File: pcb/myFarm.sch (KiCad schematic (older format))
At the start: 10 parts, among them J0 Conn_01x02, J1 LED, J2 SENSOR, J3 SW_LED, J4 RELAY, J5 POWER DRIVE, J6 JUMPER, J7 SW_LED, U1 WeMos_D1_mini, U2 MCP23017_MODULE

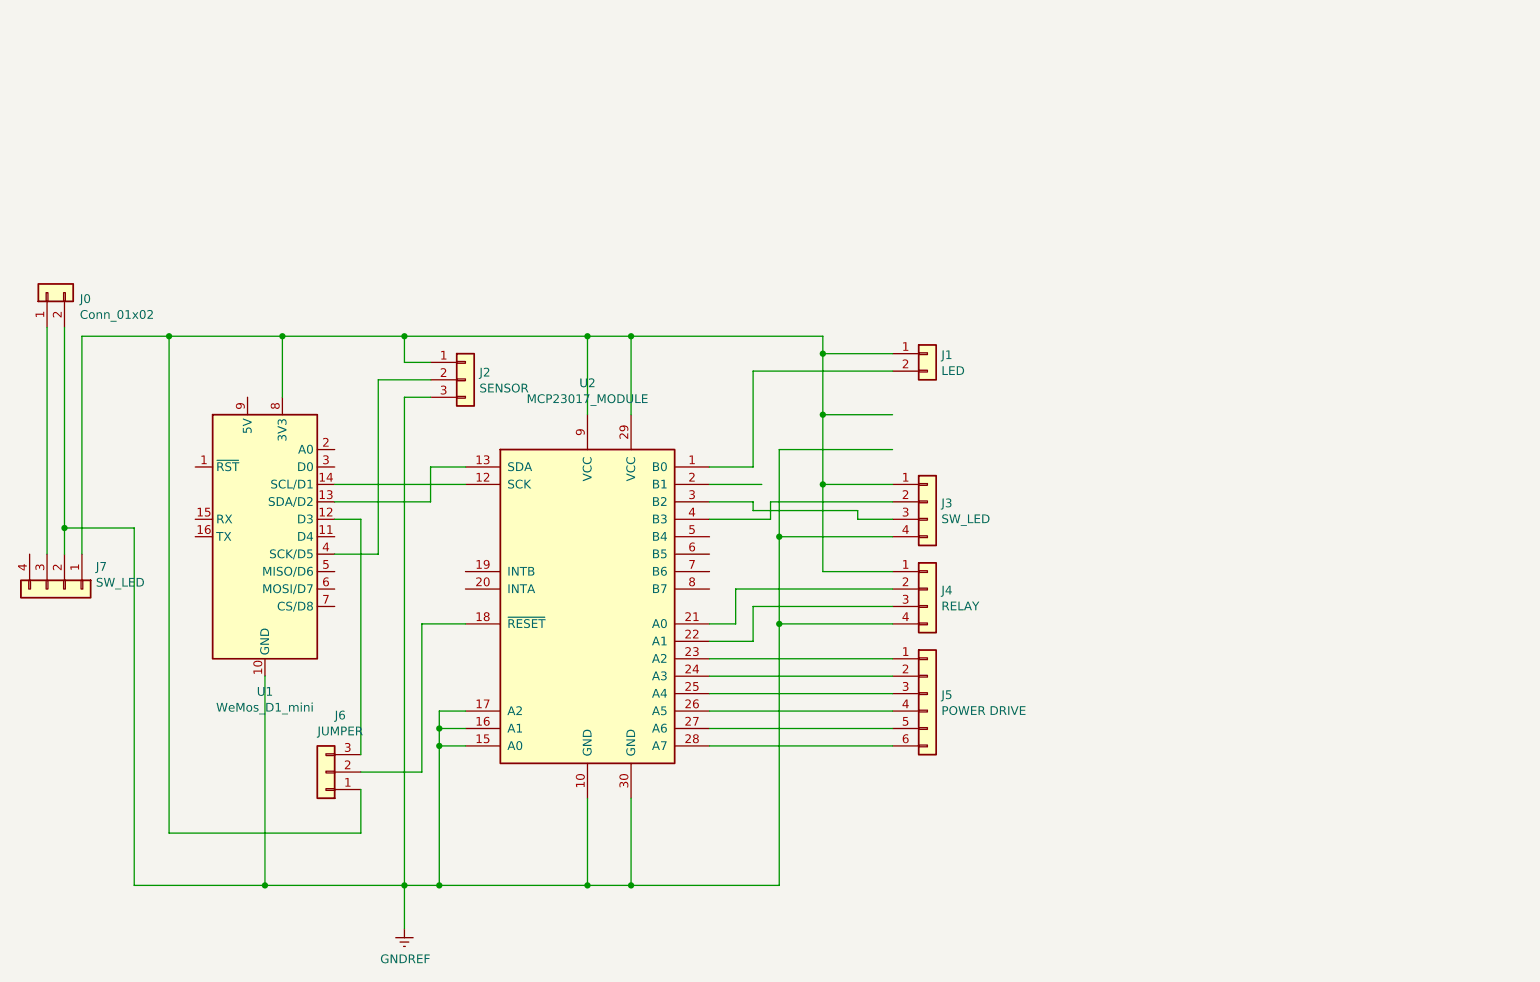
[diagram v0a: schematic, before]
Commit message: update pcb
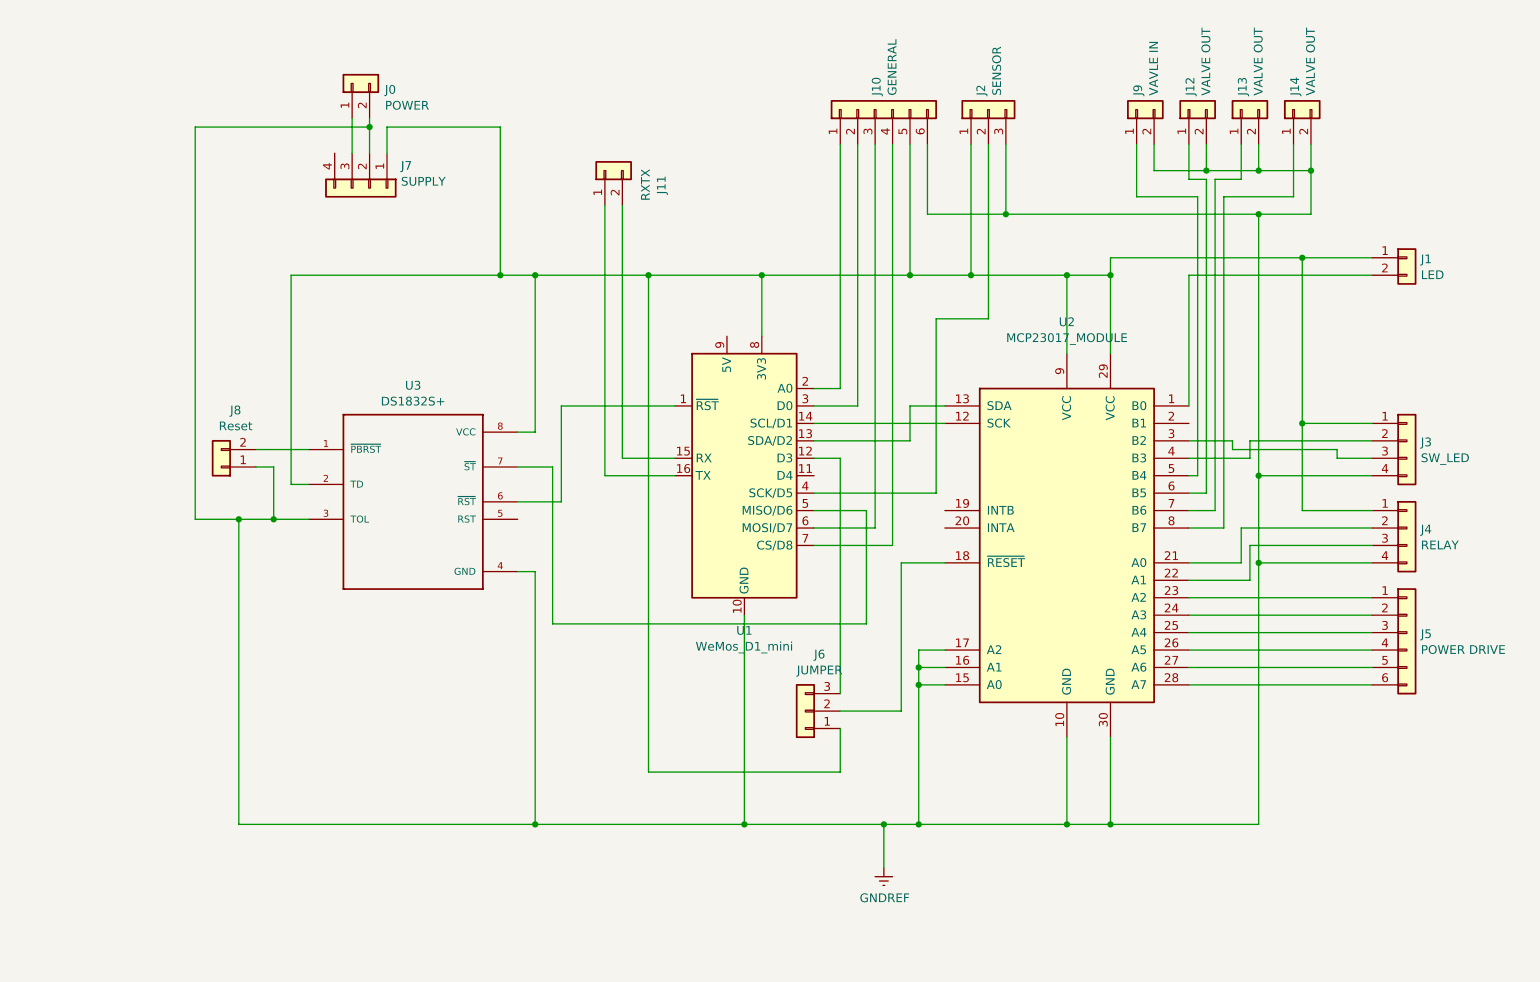
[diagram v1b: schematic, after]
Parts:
- added J10: GENERAL, Connector_PinHeader_2.54mm:PinHeader_1x06_P2.54mm_Vertical, symbol Connector_Generic:Conn_01x06
- added J11: RXTX, Connector_PinHeader_2.54mm:PinHeader_1x02_P2.54mm_Vertical, symbol Connector_Generic:Conn_01x02
- added J12, J13, J14: VALVE OUT, Connector_PinHeader_2.54mm:PinHeader_1x02_P2.54mm_Vertical, symbol Connector_Generic:Conn_01x02
- added J8: Reset, Connector_PinHeader_2.54mm:PinHeader_1x02_P2.54mm_Vertical, symbol Connector_Generic:Conn_01x02
- added J9: VAVLE IN, Connector_PinHeader_2.54mm:PinHeader_1x02_P2.54mm_Vertical, symbol Connector_Generic:Conn_01x02
- added U3: DS1832S+, Package_DIP:DIP-8_W10.16mm, symbol DS1832S_:DS1832S+
- J0: value Conn_01x02 -> POWER
- J7: value SW_LED -> SUPPLY
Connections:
- wire segments 88 -> 150
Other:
- moved on the sheet: J0, J1, J2, J3, J4, J5, J6, J7, U1, U2

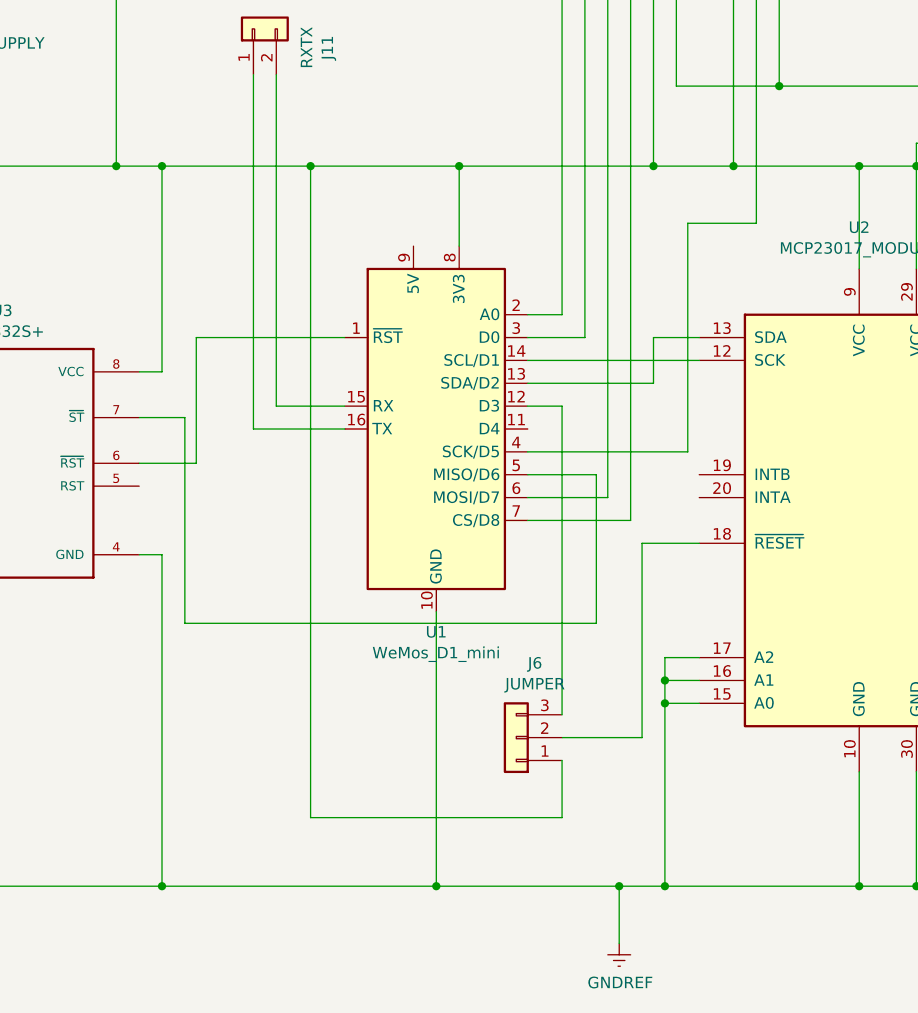
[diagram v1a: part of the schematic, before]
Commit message: update pcb.
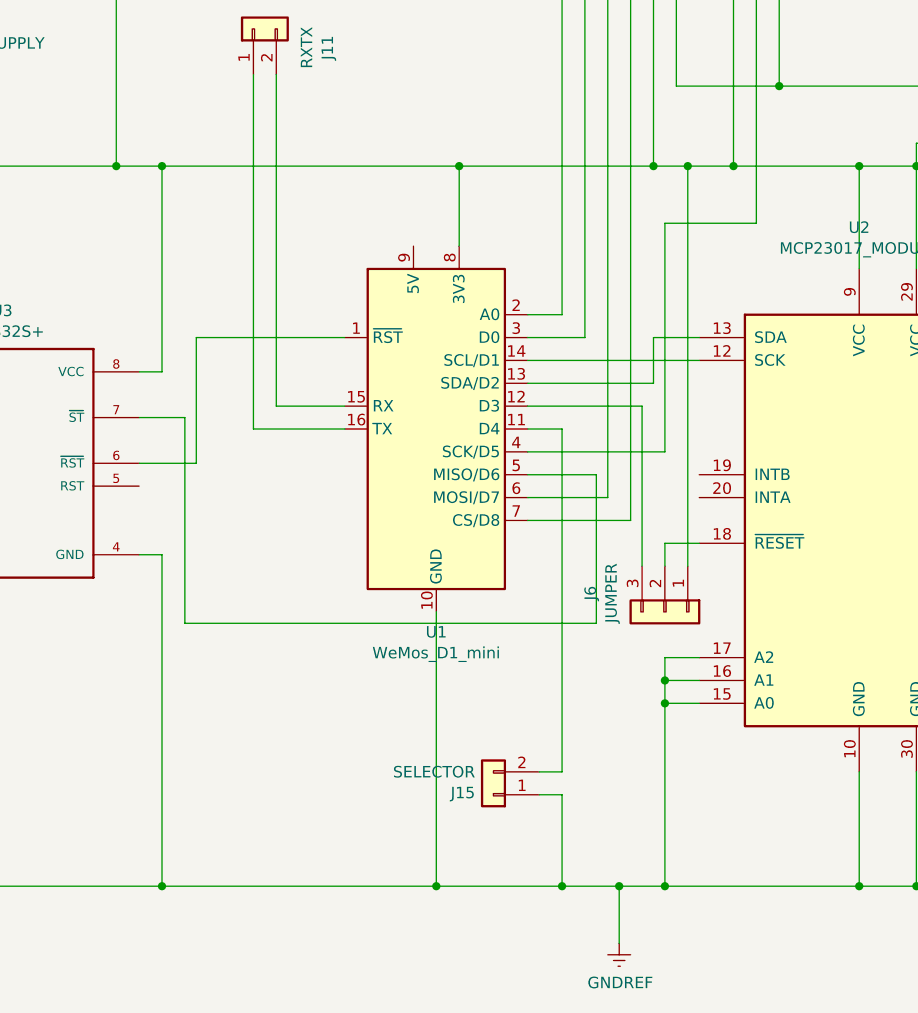
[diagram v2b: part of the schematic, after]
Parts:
- added J15: SELECTOR, Connector_PinHeader_2.54mm:PinHeader_1x02_P2.54mm_Vertical, symbol Connector_Generic:Conn_01x02
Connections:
- net GNDREF: now also J15.1 (Pin_1)
- net at U1.11 (D4): now also J15.2 (Pin_2)
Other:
- moved on the sheet: J6
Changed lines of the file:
@@
 	5450 4500 5450 5700
 Wire Wire Line
-	5450 5700 6250 5700
+	5450 5700 6000 5700
 Wire Wire Line
 	7300 5200 7300 5700
@@
 Wire Wire Line
 	7300 2550 7550 2550
-Wire Wire Line
-	5850 3600 6000 3600
-Wire Wire Line
-	6600 4200 6350 4200
 Wire Wire Line
 	6250 5950 6250 5700
@@
 	8000 4900 9050 4900
 Connection ~ 5550 2550
-$Comp
-L Connector_Generic:Conn_01x03 J6
-U 1 1 5D3BA3DB
-P 5800 5050
-F 0 "J6" H 5718 4725 50  0000 C CNN
-F 1 "JUMPER" H 5718 4816 50  0000 C CNN
-F 2 "Connector_PinHeader_2.54mm:PinHeader_1x03_P2.54mm_Vertical" H 5800 5050 50  0001 C CNN
-F 3 "~" H 5800 5050 50  0001 C CNN
-	1    5800 5050
-	-1   0    0    1
-$EndComp
-Wire Wire Line
-	6350 4200 6350 5050
-Wire Wire Line
-	6350 5050 6000 5050
-Wire Wire Line
-	6000 5150 6000 5400
-Wire Wire Line
-	6000 5400 4900 5400
-Wire Wire Line
-	4900 2550 5550 2550
-Wire Wire Line
-	4900 5400 4900 2550
 Wire Wire Line
 	8000 3600 8350 3600
@@
 Wire Wire Line
 	3400 1700 4050 1700
-Connection ~ 4900 2550
 Wire Wire Line
 	4250 4250 4250 5700
@@
 Wire Wire Line
 	4250 3450 4250 2550
-Wire Wire Line
-	4250 2550 4900 2550
 Wire Wire Line
 	4400 3850 4400 3300
@@
 Wire Wire Line
 	3300 1700 3300 1850
-Wire Wire Line
-	6000 3600 6000 4950
 Wire Wire Line
 	5850 3900 6150 3900
@@
 	6850 2800 6850 1800
 Wire Wire Line
-	6550 3800 6550 2800
-Wire Wire Line
-	6550 2800 6850 2800
-Wire Wire Line
-	5850 3800 6550 3800
+	6450 3800 6450 2800
+Wire Wire Line
+	6450 2800 6850 2800
+Wire Wire Line
+	5850 3800 6450 3800
 Wire Wire Line
 	6000 1800 6000 3200
@@
 Connection ~ 6400 2550
 Wire Wire Line
-	6400 2550 6750 2550
+	6400 2550 6550 2550
 Wire Wire Line
 	6500 1800 6500 2200
@@
 	8650 2450 9050 2450
 $Comp
+L Connector_Generic:Conn_01x02 J9
+U 1 1 5D6744E9
+P 7700 1600
+F 0 "J9" H 7780 1592 50  0000 L CNN
+F 1 "VAVLE IN" H 7780 1501 50  0000 L CNN
+F 2 "Connector_PinHeader_2.54mm:PinHeader_1x02_P2.54mm_Vertical" H 7700 1600 50  0001 C CNN
+F 3 "~" H 7700 1600 50  0001 C CNN
+	1    7700 1600
+	0    -1   -1   0
+$EndComp
+$Comp
+L Connector_Generic:Conn_01x02 J12
+U 1 1 5D67486F
+P 8000 1600
+F 0 "J12" H 8080 1592 50  0000 L CNN
+F 1 "VALVE OUT" H 8080 1501 50  0000 L CNN
+F 2 "Connector_PinHeader_2.54mm:PinHeader_1x02_P2.54mm_Vertical" H 8000 1600 50  0001 C CNN
+F 3 "~" H 8000 1600 50  0001 C CNN
+	1    8000 1600
+	0    -1   -1   0
+$EndComp
+$Comp
+L Connector_Generic:Conn_01x02 J13
+U 1 1 5D6923CB
+P 8300 1600
+F 0 "J13" H 8380 1592 50  0000 L CNN
+F 1 "VALVE OUT" H 8380 1501 50  0000 L CNN
+F 2 "Connector_PinHeader_2.54mm:PinHeader_1x02_P2.54mm_Vertical" H 8300 1600 50  0001 C CNN
+F 3 "~" H 8300 1600 50  0001 C CNN
+	1    8300 1600
+	0    -1   -1   0
+$EndComp
+$Comp
+L Connector_Generic:Conn_01x02 J14
+U 1 1 5D692989
+P 8600 1600
+F 0 "J14" H 8680 1592 50  0000 L CNN
+F 1 "VALVE OUT" H 8680 1501 50  0000 L CNN
+F 2 "Connector_PinHeader_2.54mm:PinHeader_1x02_P2.54mm_Vertical" H 8600 1600 50  0001 C CNN
+F 3 "~" H 8600 1600 50  0001 C CNN
+	1    8600 1600
+	0    -1   -1   0
+$EndComp
+Wire Wire Line
+	8050 2100 7700 2100
+Wire Wire Line
+	7700 2100 7700 1800
+Wire Wire Line
+	8050 2100 8050 3700
+Wire Wire Line
+	8100 2000 8000 2000
+Wire Wire Line
+	8000 2000 8000 1800
+Wire Wire Line
+	8100 2000 8100 3800
+Wire Wire Line
+	8150 2000 8300 2000
+Wire Wire Line
+	8300 2000 8300 1800
+Wire Wire Line
+	8150 2000 8150 3900
+Wire Wire Line
+	8200 2100 8600 2100
+Wire Wire Line
+	8600 2100 8600 1800
+Wire Wire Line
+	8200 2100 8200 4000
+Wire Wire Line
+	7800 1800 7800 1950
+Wire Wire Line
+	7800 1950 8100 1950
+Wire Wire Line
+	8700 1950 8700 2200
+Wire Wire Line
+	8700 2200 8400 2200
+Connection ~ 8400 2200
+Wire Wire Line
+	8700 1800 8700 1950
+Connection ~ 8700 1950
+Wire Wire Line
+	8400 1800 8400 1950
+Connection ~ 8400 1950
+Wire Wire Line
+	8400 1950 8700 1950
+Wire Wire Line
+	8100 1800 8100 1950
+Connection ~ 8100 1950
+Wire Wire Line
+	8100 1950 8400 1950
+$Comp
+L Connector_Generic:Conn_01x03 J6
+U 1 1 5D3BA3DB
+P 6450 4500
+F 0 "J6" H 6368 4175 50  0000 C CNN
+F 1 "JUMPER" H 6368 4266 50  0000 C CNN
+F 2 "Connector_PinHeader_2.54mm:PinHeader_1x03_P2.54mm_Vertical" H 6450 4500 50  0001 C CNN
+F 3 "~" H 6450 4500 50  0001 C CNN
+	1    6450 4500
+	0    1    1    0
+$EndComp
+Wire Wire Line
+	6600 4200 6450 4200
+Wire Wire Line
+	6450 4200 6450 4300
+Wire Wire Line
+	6350 3600 6350 4300
+Wire Wire Line
+	6550 4300 6550 2550
+Connection ~ 6550 2550
+Wire Wire Line
+	6550 2550 6750 2550
+Wire Wire Line
+	5850 3600 6350 3600
+Wire Wire Line
+	4250 2550 5550 2550
+$Comp
+L Connector_Generic:Conn_01x02 J15
+U 1 1 5D75F2CC
+P 5700 5300
+F 0 "J15" H 5780 5292 50  0000 L CNN
+F 1 "SELECTOR" H 5780 5201 50  0000 L CNN
+F 2 "Connector_PinHeader_2.54mm:PinHeader_1x02_P2.54mm_Vertical" H 5700 5300 50  0001 C CNN
+F 3 "~" H 5700 5300 50  0001 C CNN
+	1    5700 5300
+	-1   0    0    1
+$EndComp
+Wire Wire Line
+	5850 3700 6000 3700
+Wire Wire Line
+	6000 3700 6000 5200
+Wire Wire Line
+	6000 5200 5900 5200
+Wire Wire Line
+	5900 5300 6000 5300
+Wire Wire Line
+	6000 5300 6000 5700
+Connection ~ 6000 5700
+Wire Wire Line
+	6000 5700 6250 5700
+$Comp
 L Connector_Generic:Conn_01x02 J1
 U 1 1 5D3273EB
@@
 	1    0    0    -1
 $EndComp
-$Comp
-L Connector_Generic:Conn_01x02 J9
-U 1 1 5D6744E9
-P 7700 1600
-F 0 "J9" H 7780 1592 50  0000 L CNN
-F 1 "VAVLE IN" H 7780 1501 50  0000 L CNN
-F 2 "Connector_PinHeader_2.54mm:PinHeader_1x02_P2.54mm_Vertical" H 7700 1600 50  0001 C CNN
-F 3 "~" H 7700 1600 50  0001 C CNN
-	1    7700 1600
-	0    -1   -1   0
-$EndComp
-$Comp
-L Connector_Generic:Conn_01x02 J12
-U 1 1 5D67486F
-P 8000 1600
-F 0 "J12" H 8080 1592 50  0000 L CNN
-F 1 "VALVE OUT" H 8080 1501 50  0000 L CNN
-F 2 "Connector_PinHeader_2.54mm:PinHeader_1x02_P2.54mm_Vertical" H 8000 1600 50  0001 C CNN
-F 3 "~" H 8000 1600 50  0001 C CNN
-	1    8000 1600
-	0    -1   -1   0
-$EndComp
-$Comp
-L Connector_Generic:Conn_01x02 J13
-U 1 1 5D6923CB
-P 8300 1600
-F 0 "J13" H 8380 1592 50  0000 L CNN
-F 1 "VALVE OUT" H 8380 1501 50  0000 L CNN
-F 2 "Connector_PinHeader_2.54mm:PinHeader_1x02_P2.54mm_Vertical" H 8300 1600 50  0001 C CNN
-F 3 "~" H 8300 1600 50  0001 C CNN
-	1    8300 1600
-	0    -1   -1   0
-$EndComp
-$Comp
-L Connector_Generic:Conn_01x02 J14
-U 1 1 5D692989
-P 8600 1600
-F 0 "J14" H 8680 1592 50  0000 L CNN
-F 1 "VALVE OUT" H 8680 1501 50  0000 L CNN
-F 2 "Connector_PinHeader_2.54mm:PinHeader_1x02_P2.54mm_Vertical" H 8600 1600 50  0001 C CNN
-F 3 "~" H 8600 1600 50  0001 C CNN
-	1    8600 1600
-	0    -1   -1   0
-$EndComp
-Wire Wire Line
-	8050 2100 7700 2100
-Wire Wire Line
-	7700 2100 7700 1800
-Wire Wire Line
-	8050 2100 8050 3700
-Wire Wire Line
-	8100 2000 8000 2000
-Wire Wire Line
-	8000 2000 8000 1800
-Wire Wire Line
-	8100 2000 8100 3800
-Wire Wire Line
-	8150 2000 8300 2000
-Wire Wire Line
-	8300 2000 8300 1800
-Wire Wire Line
-	8150 2000 8150 3900
-Wire Wire Line
-	8200 2100 8600 2100
-Wire Wire Line
-	8600 2100 8600 1800
-Wire Wire Line
-	8200 2100 8200 4000
-Wire Wire Line
-	7800 1800 7800 1950
-Wire Wire Line
-	7800 1950 8100 1950
-Wire Wire Line
-	8700 1950 8700 2200
-Wire Wire Line
-	8700 2200 8400 2200
-Connection ~ 8400 2200
-Wire Wire Line
-	8700 1800 8700 1950
-Connection ~ 8700 1950
-Wire Wire Line
-	8400 1800 8400 1950
-Connection ~ 8400 1950
-Wire Wire Line
-	8400 1950 8700 1950
-Wire Wire Line
-	8100 1800 8100 1950
-Connection ~ 8100 1950
-Wire Wire Line
-	8100 1950 8400 1950
 $EndSCHEMATC
